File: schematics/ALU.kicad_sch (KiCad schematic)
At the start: 12 parts, among them U10 74LS173, U11 74LS243, U8 74LS86, U9 74LS283

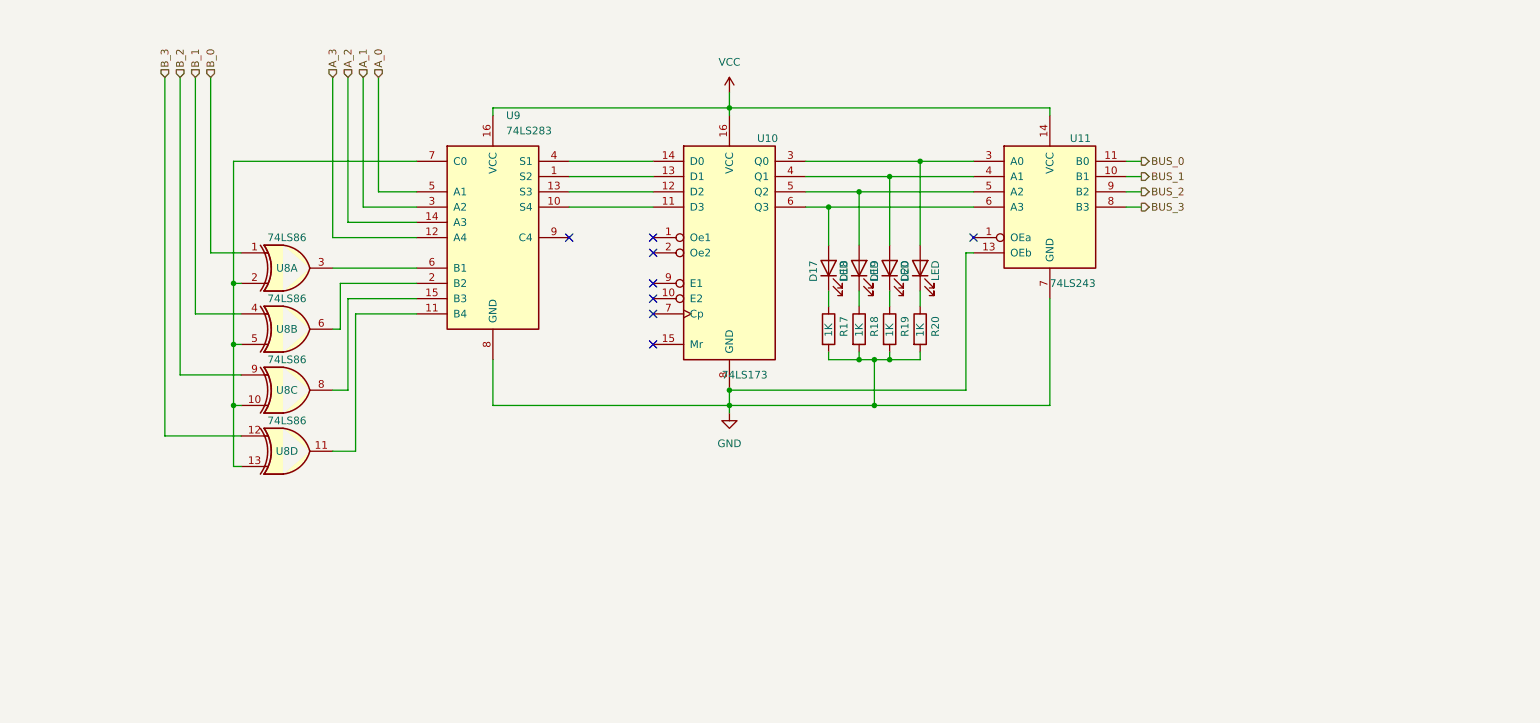
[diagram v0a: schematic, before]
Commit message: lesson5
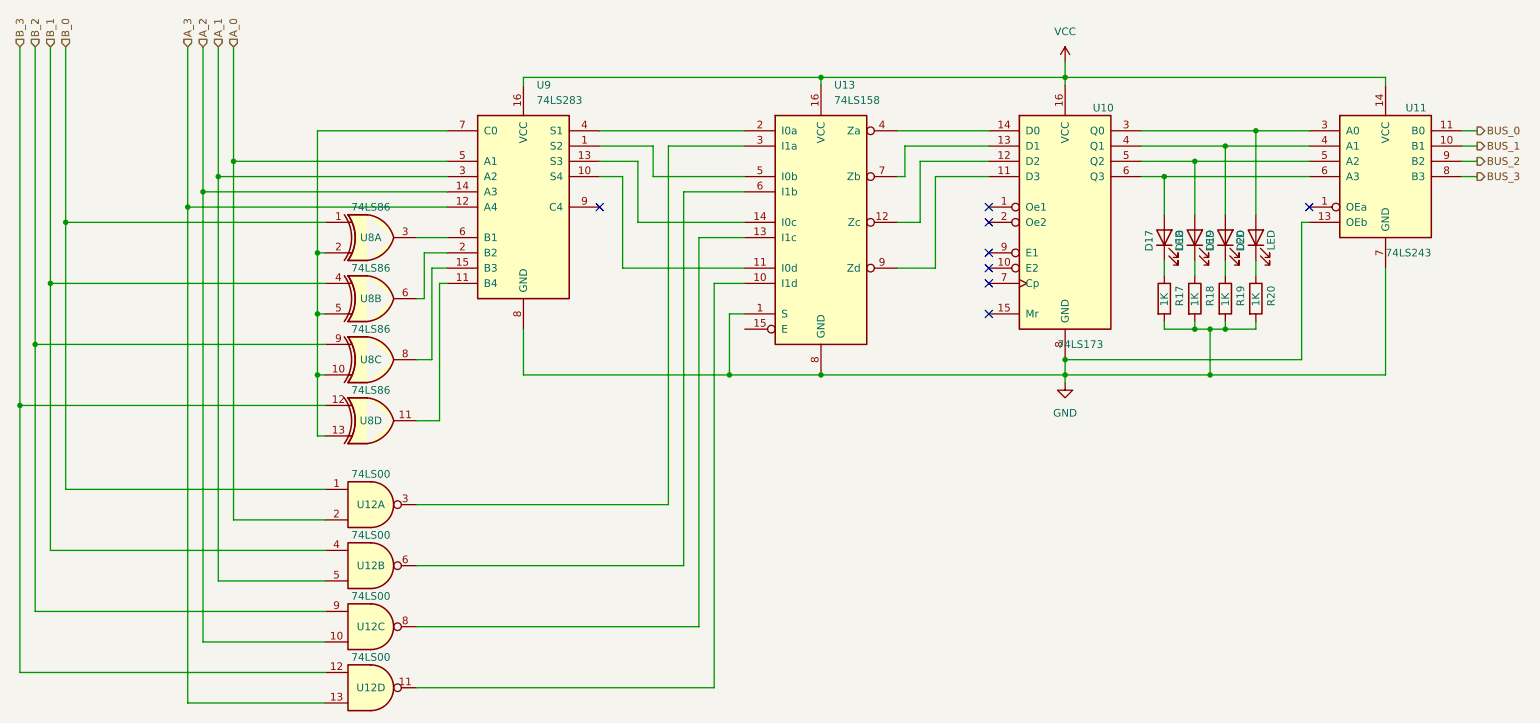
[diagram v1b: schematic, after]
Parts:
- added U12: 74LS00, symbol 74xx:74LS00
- added U13: 74LS158, symbol 74xx:74LS158
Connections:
- net A_0: now also U12.2
- net A_1: now also U12.5
- net A_2: now also U12.10
- net A_3: now also U12.13
- net B_0: now also U12.1
- net B_1: now also U12.4
- net B_2: now also U12.9
- net B_3: now also U12.12
- net GND: now also U13.1 (S), U13.8 (GND)
- net VCC: now also U13.16 (VCC)
- net at U9.10 (S4): now also U13.11 (I0d); no longer U10.11 (D3)
- net at U10.12 (D2): now also U13.12 (Zc); no longer U9.13 (S3)
- net at U9.1 (S2): now also U13.5 (I0b); no longer U10.13 (D1)
- net at U9.4 (S1): now also U13.2 (I0a); no longer U10.14 (D0)
- new net: U12.8, U13.13 (I1c)
- new net: U12.11, U13.10 (I1d)
- new net: U13.14 (I0c), U9.13 (S3)
- new net: U12.3, U13.3 (I1a)
- new net: U10.14 (D0), U13.4 (Za)
- new net: U12.6, U13.6 (I1b)
- new net: U10.13 (D1), U13.7 (Zb)
- new net: U10.11 (D3), U13.9 (Zd)
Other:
- moved on the sheet: D17, D18, D19, D20, R17, R18, R19, R20, U10, U11, U8A, U8B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
